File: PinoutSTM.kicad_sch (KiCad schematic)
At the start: 12 parts, among them IC1 STM32H7B0RBT6, J4 1761681-3, J6 Header male 1x05, SW1 Button Switch SPST-No, Y1 CC4V-T1A-32.768kHz-6pF-20PPM-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

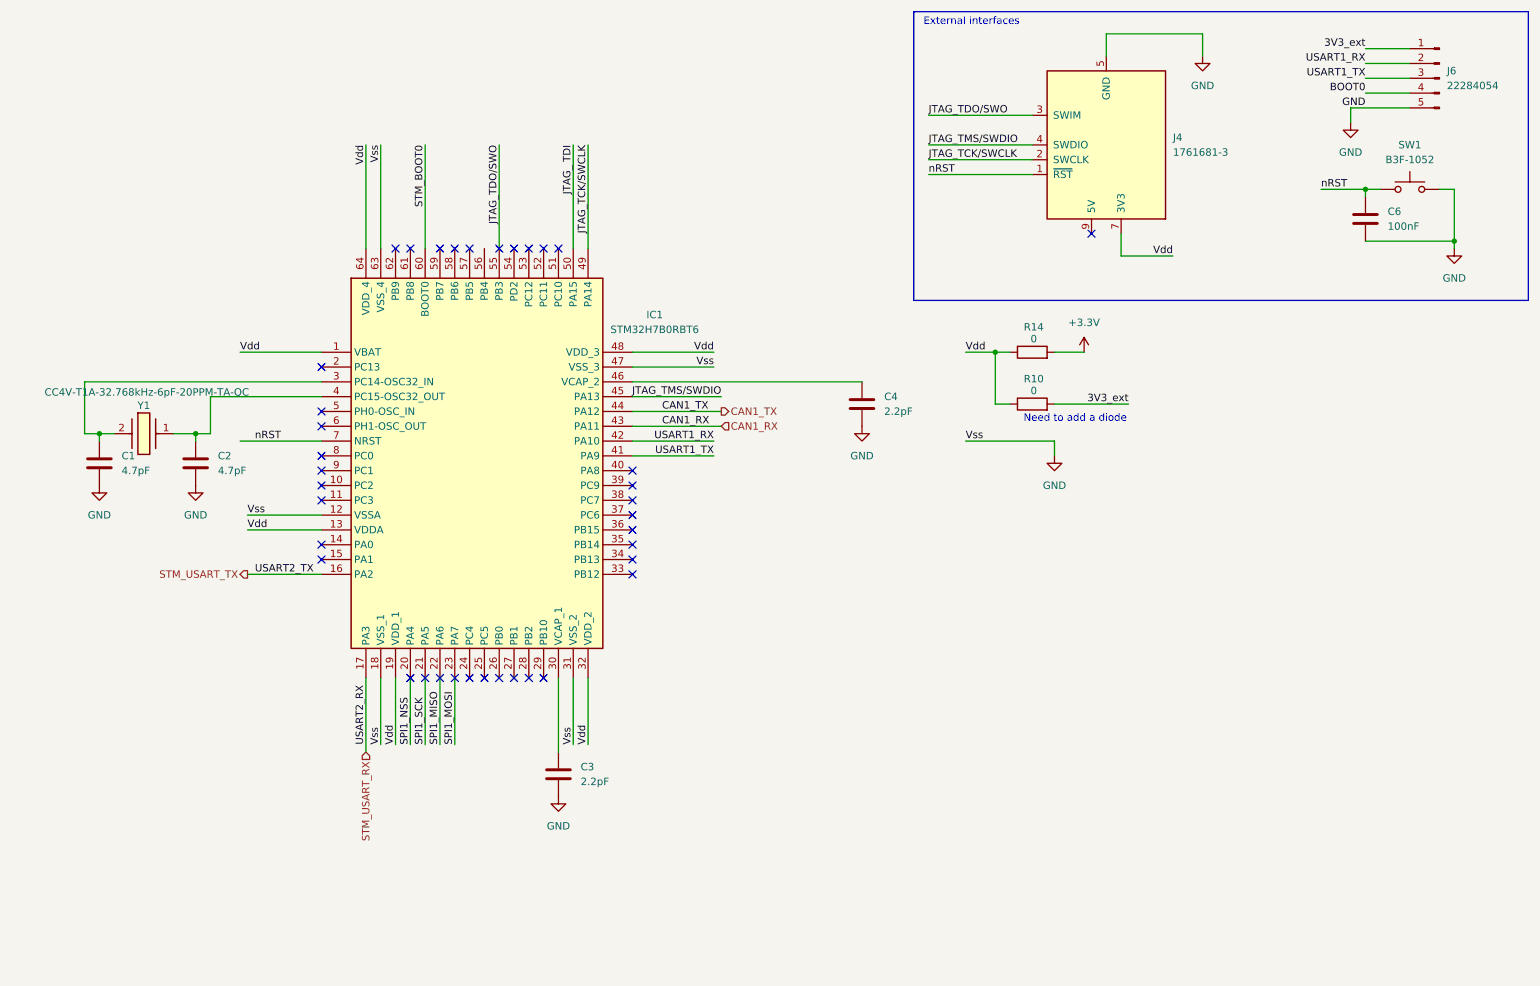
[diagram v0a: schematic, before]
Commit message: added caps
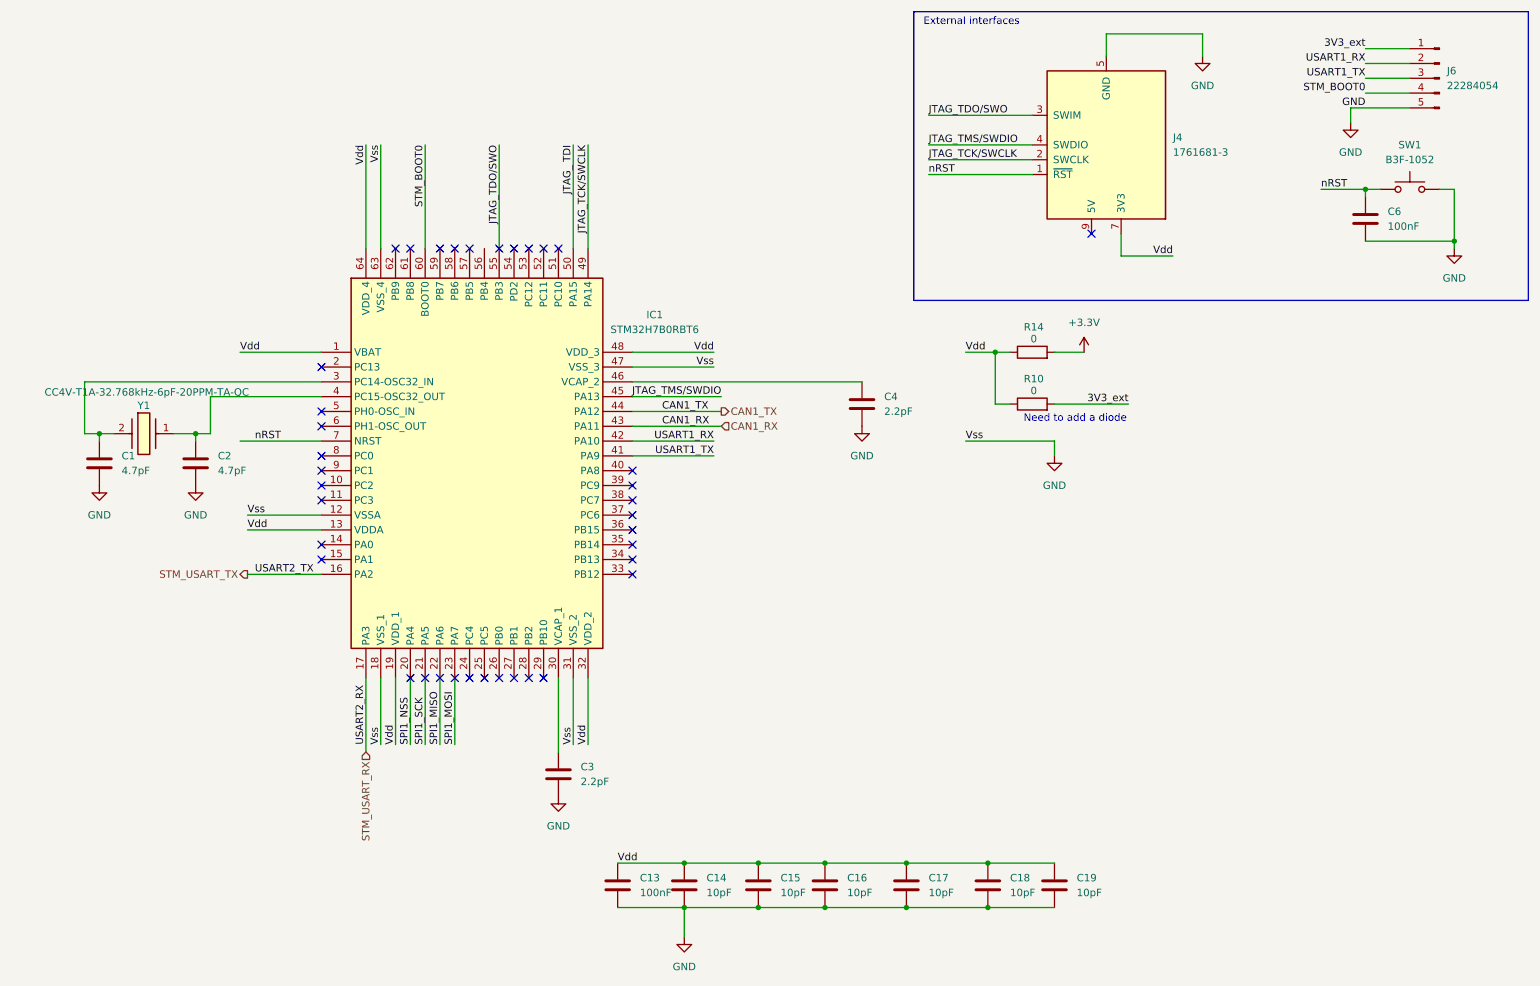
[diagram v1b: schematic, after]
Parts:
- added C13: 100nF, Capacitor_SMD:C_0603_1608Metric, symbol #dzdb:g_cap/C-100n-0603
- added C14, C15, C16, C17, C18, C19: 10pF, Capacitor_SMD:C_0603_1608Metric, symbol #dzdb:g_cap/C-10p-0603
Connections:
- net BOOT0 is gone; now on net STM_BOOT0: J6.4 (Pin_4)
- net GND: now also C13.2, C14.2, C15.2, C16.2, C17.2, C18.2, C19.2
- net Vdd: now also C13.1, C14.1, C15.1, C16.1, C17.1, C18.1, C19.1
